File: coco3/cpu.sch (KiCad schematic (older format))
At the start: 15 parts, among them IC1 MC6809E, IC3 SN74LS245N, SW2 Reset Switch

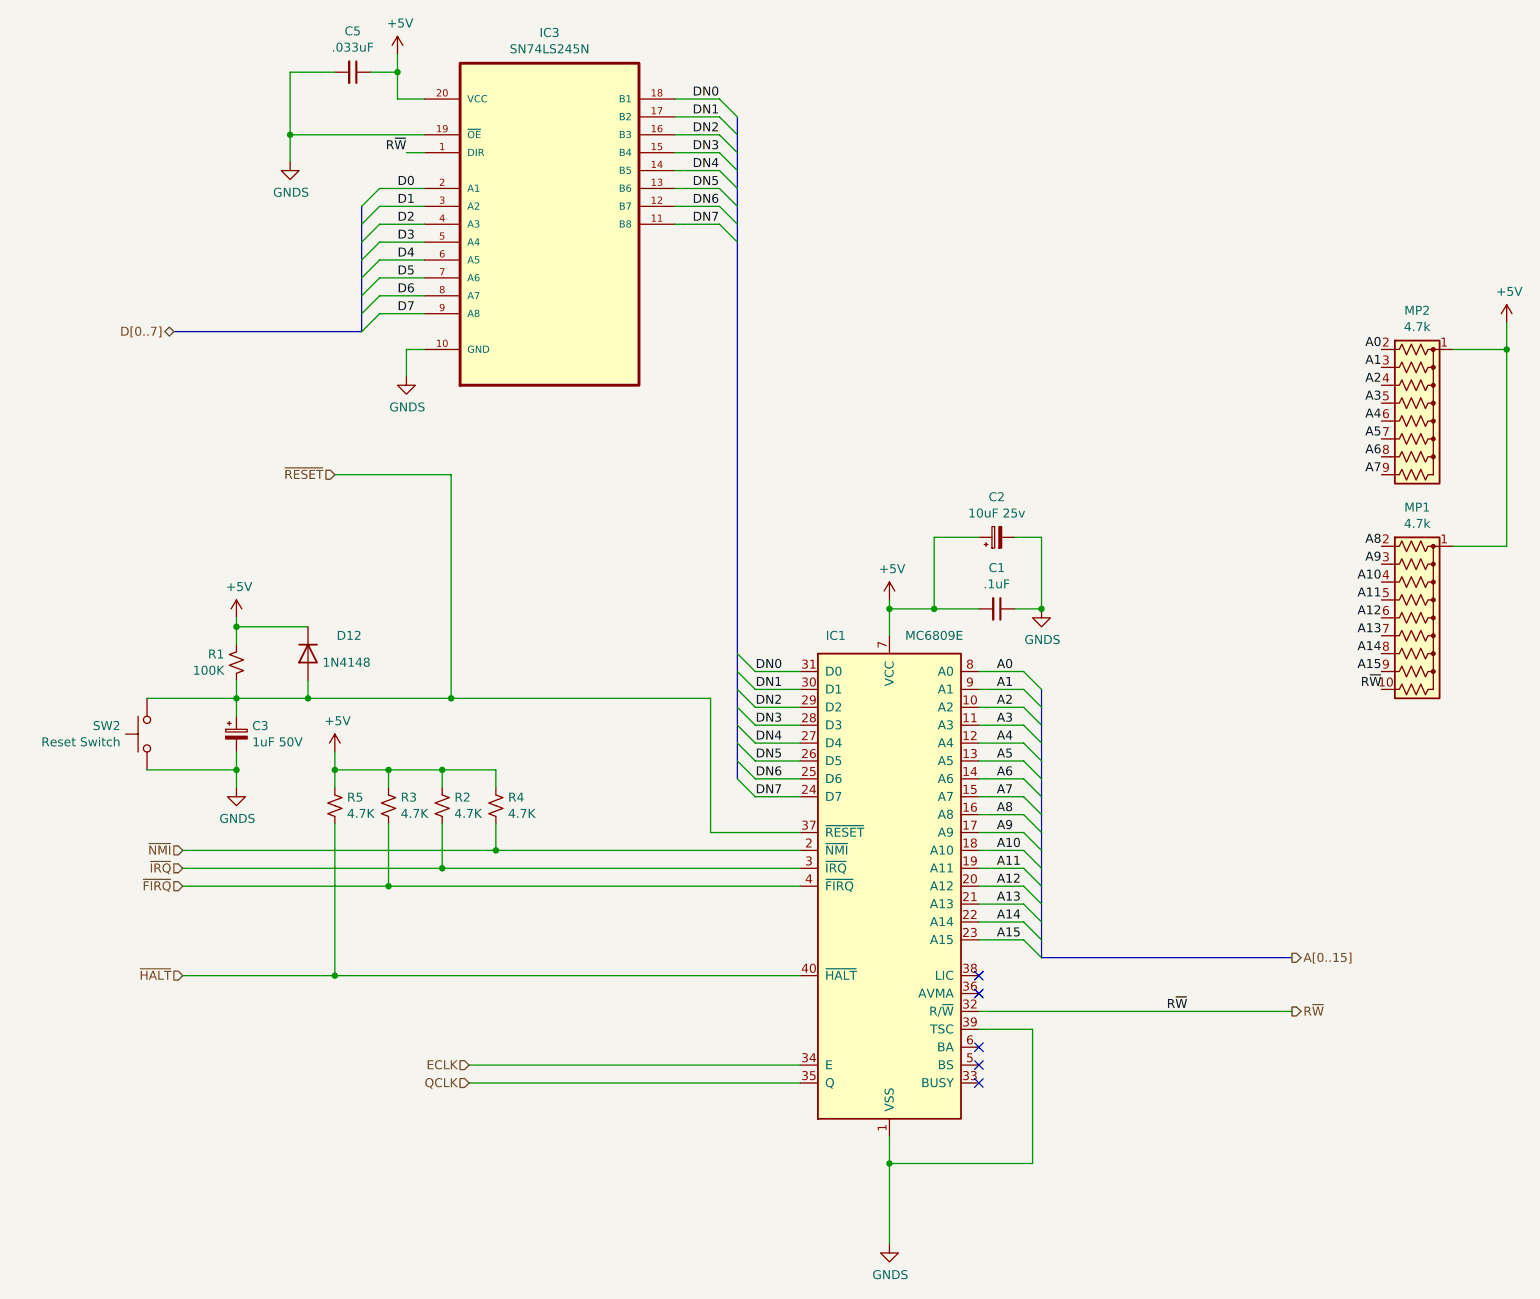
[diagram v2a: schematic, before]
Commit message: routed the board
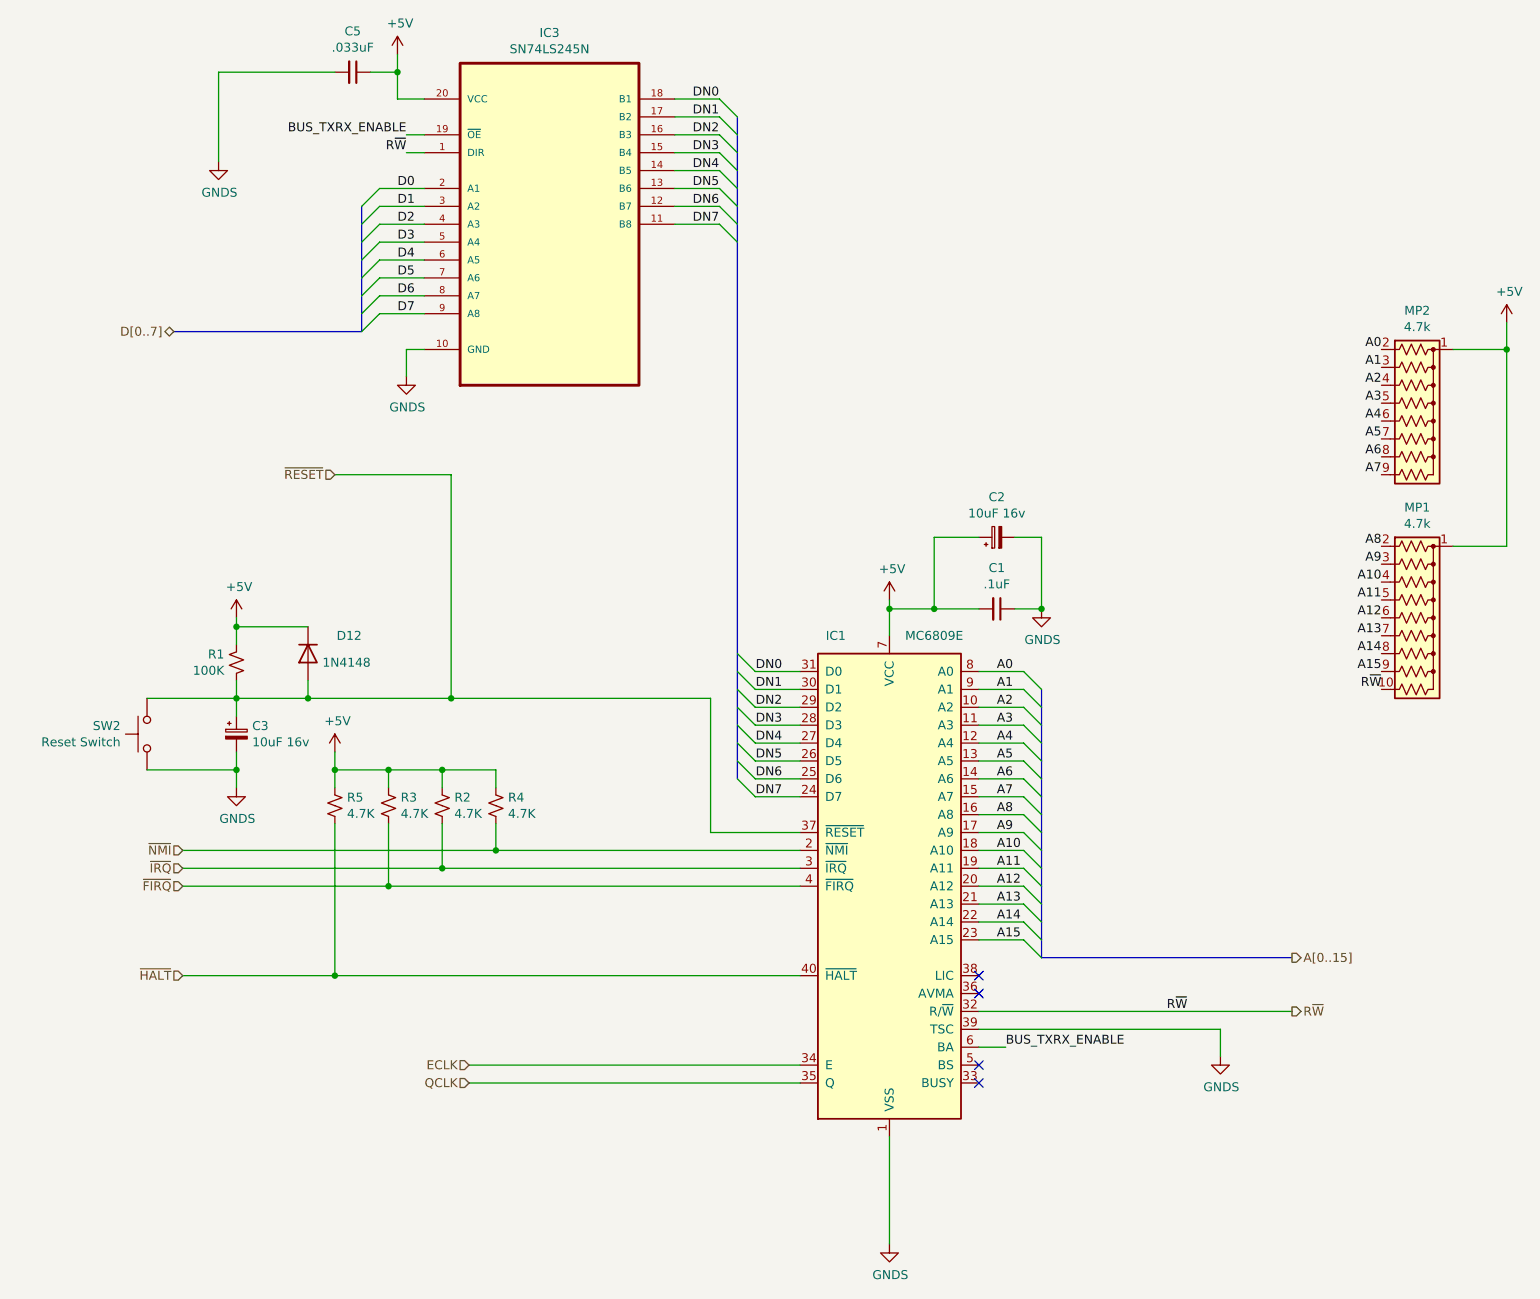
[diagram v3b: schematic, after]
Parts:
- C2: value 10uF 25v -> 10uF 16v; footprint Capacitor_SMD:CP_Elec_4x5.3 -> Capacitor_Tantalum_SMD:CP_EIA-3216-18_Kemet-A; Manufacturer part# VE-100M1ETR-0405 -> TAJA106K016RNJ; Vendor part# C134721 -> C7171
- C3: value 1uF 50V -> 10uF 16v; footprint Capacitor_SMD:CP_Elec_4x5.4 -> Capacitor_Tantalum_SMD:CP_EIA-3216-18_Kemet-A; Manufacturer part# RVT1H1R0M0405 -> TAJA106K016RNJ; Vendor part# C3348 -> C7171
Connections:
- net GNDS: no longer IC3.19 (~OE)
- net BUS_TXRX_ENABLE: now reaches IC1.6 (BA)
- net BUS_TXRX_ENABLE: now also IC3.19 (~OE)
- no-connect marks 5 -> 4
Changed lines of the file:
@@
 $EndComp
 NoConn ~ 5800 6550
-NoConn ~ 5800 6450
 NoConn ~ 5800 6150
 NoConn ~ 5800 6050
@@
 	1    0    0    -1
 $EndComp
-Wire Wire Line
-	5300 6950 5300 7100
 $Comp
 L power:+5V #PWR01027
@@
 	2700 2350 2450 2350
 Wire Wire Line
-	5800 6350 6100 6350
-Wire Wire Line
-	6100 6350 6100 7100
-Wire Wire Line
-	6100 7100 5300 7100
-Connection ~ 5300 7100
-Wire Wire Line
 	4800 5250 4300 5250
 Wire Wire Line
@@
 AR Path="/60273794/60456BFE" Ref="C3"  Part="1"
 F 0 "C3" H 1738 4746 50  0000 L CNN
-F 1 "1uF 50V" H 1738 4655 50  0000 L CNN
-F 2 "Capacitor_SMD:CP_Elec_4x5.4" H 1650 4700 50  0001 C CNN
-F 3 " https://datasheet.lcsc.com/lcsc/2105211834_Honor-Elec-RVT1H1R0M0405_C3348.pdf" H 1650 4700 50  0001 C CNN
+F 1 "10uF 16v" H 1738 4655 50  0000 L CNN
+F 2 "Capacitor_Tantalum_SMD:CP_EIA-3216-18_Kemet-A" H 1650 4700 50  0001 C CNN
+F 3 "https://datasheet.lcsc.com/lcsc/1811071223_AVX-TAJA106K016RNJ_C7171.pdf" H 1650 4700 50  0001 C CNN
 F 4 "JLCPCB" H 1650 4700 50  0001 C CNN "Vendor"
-F 5 "C3348" H 1650 4700 50  0001 C CNN "Vendor part#"
-F 6 "RVT1H1R0M0405" H 1650 4700 50  0001 C CNN "Manufacturer part#"
+F 5 "C7171" H 1650 4700 50  0001 C CNN "Vendor part#"
+F 6 "TAJA106K016RNJ" H 1650 4700 50  0001 C CNN "Manufacturer part#"
 	1    1650 4700
 	1    0    0    -1
@@
 P 5900 3600
 F 0 "C2" V 6125 3600 50  0000 C CNN
-F 1 "10uF 25v" V 6034 3600 50  0000 C CNN
-F 2 "Capacitor_SMD:CP_Elec_4x5.3" H 5900 3600 50  0001 C CNN
-F 3 "https://datasheet.lcsc.com/lcsc/1809291326_Lelon-VE-100M1ETR-0405_C134721.pdf" H 5900 3600 50  0001 C CNN
+F 1 "10uF 16v" V 6034 3600 50  0000 C CNN
+F 2 "Capacitor_Tantalum_SMD:CP_EIA-3216-18_Kemet-A" H 5900 3600 50  0001 C CNN
+F 3 "https://datasheet.lcsc.com/lcsc/1811071223_AVX-TAJA106K016RNJ_C7171.pdf" H 5900 3600 50  0001 C CNN
 F 4 "JLCPCB" V 5900 3600 50  0001 C CNN "Vendor"
-F 5 "C134721" V 5900 3600 50  0001 C CNN "Vendor part#"
-F 6 "VE-100M1ETR-0405" V 5900 3600 50  0001 C CNN "Manufacturer part#"
+F 5 "C7171" V 5900 3600 50  0001 C CNN "Vendor part#"
+F 6 "TAJA106K016RNJ" V 5900 3600 50  0001 C CNN "Manufacturer part#"
 	1    5900 3600
 	0    -1   -1   0
@@
 	2950 6550 4800 6550
 Wire Wire Line
-	5300 7100 5300 7550
-Wire Wire Line
 	2950 6650 4800 6650
 $Comp
@@
 L power:GNDS #PWR01024
 U 1 1 61507CAC
-P 1950 1500
-F 0 "#PWR01024" H 1950 1250 50  0001 C CNN
-F 1 "GNDS" H 1955 1327 50  0000 C CNN
-F 2 "" H 1950 1500 50  0001 C CNN
-F 3 "" H 1950 1500 50  0001 C CNN
-	1    1950 1500
-	1    0    0    -1
-$EndComp
-Wire Wire Line
-	2700 1350 1950 1350
+P 1550 1500
+F 0 "#PWR01024" H 1550 1250 50  0001 C CNN
+F 1 "GNDS" H 1555 1327 50  0000 C CNN
+F 2 "" H 1550 1500 50  0001 C CNN
+F 3 "" H 1550 1500 50  0001 C CNN
+	1    1550 1500
+	1    0    0    -1
+$EndComp
 $Comp
 L Device:C_Small C?
@@
 $EndComp
 Wire Wire Line
-	2200 1000 1950 1000
-Wire Wire Line
-	1950 1000 1950 1350
-Connection ~ 1950 1350
-Wire Wire Line
-	1950 1350 1950 1500
-Wire Wire Line
 	2400 1000 2550 1000
 Connection ~ 2550 1000
@@
 Wire Wire Line
 	1150 4500 1650 4500
+Wire Wire Line
+	1550 1000 1550 1500
+Text Label 5950 6450 0    50   ~ 0
+BUS_TXRX_ENABLE
+Wire Wire Line
+	5950 6450 5800 6450
+Wire Wire Line
+	5300 6950 5300 7550
+$Comp
+L power:GNDS #PWR0106
+U 1 1 6199B2E5
+P 7150 6500
+F 0 "#PWR0106" H 7150 6250 50  0001 C CNN
+F 1 "GNDS" H 7155 6327 50  0000 C CNN
+F 2 "" H 7150 6500 50  0001 C CNN
+F 3 "" H 7150 6500 50  0001 C CNN
+	1    7150 6500
+	1    0    0    -1
+$EndComp
+Wire Wire Line
+	7150 6350 7150 6500
+Wire Wire Line
+	5800 6350 7150 6350
+Text Label 2600 1350 2    50   ~ 0
+BUS_TXRX_ENABLE
+Wire Wire Line
+	1550 1000 2200 1000
+Wire Wire Line
+	2700 1350 2600 1350
 Wire Bus Line
 	2350 1750 2350 2450
